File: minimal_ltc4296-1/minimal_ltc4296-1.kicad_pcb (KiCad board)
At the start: 4 copper layers, 71.1 x 53.3 mm, 44 parts, among them J1 TBP02R1-381-03BE, J2 TBP02R1-381-03BE, J3 TBP02R1-381-03BE, J4 TBP02R1-381-03BE, J5 TBP02R1-381-03BE, J6 TBP02R1-381-02BE, Q1 100.0 V, Q2 100.0 V, Q3 100.0 V, Q4 100.0 V, Q5 100.0 V, Q6 100.0 V, U1 LTC4296AUK-1-PBF

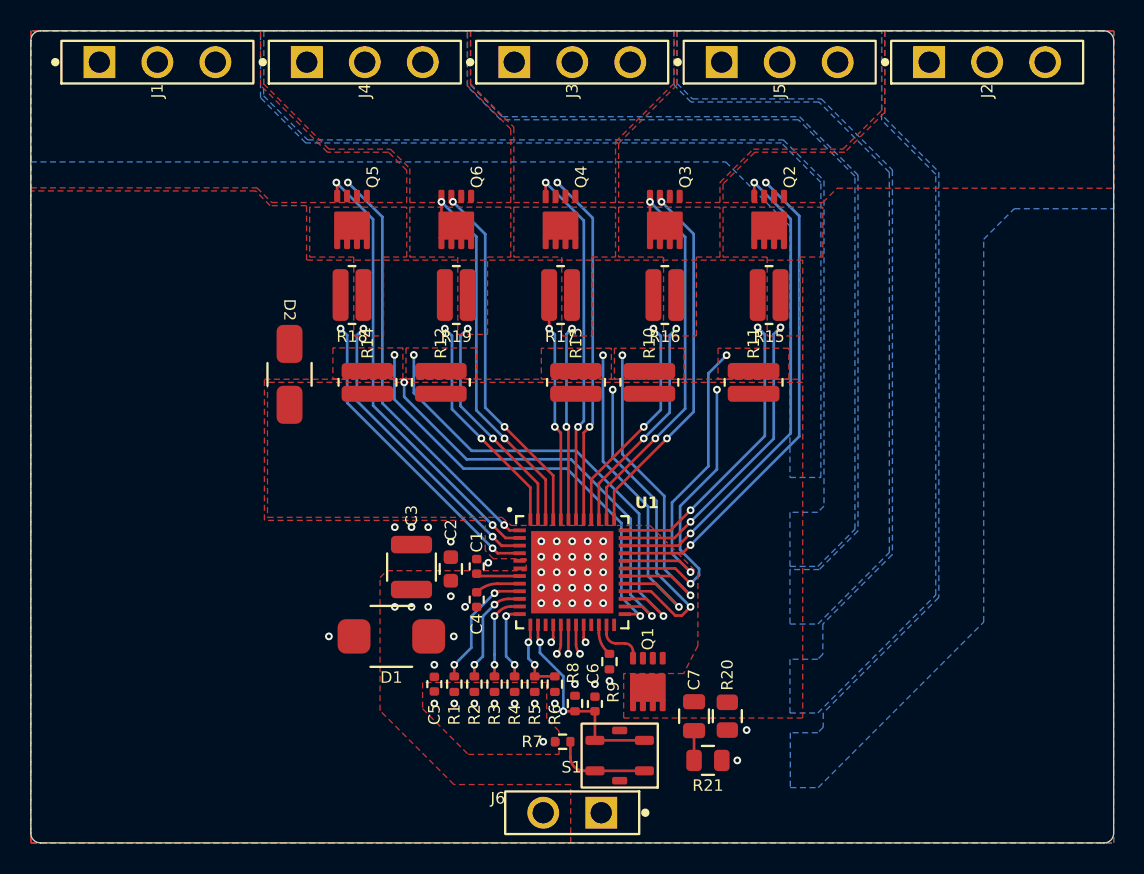
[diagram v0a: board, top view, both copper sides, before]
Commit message: Update KiCad PCB file
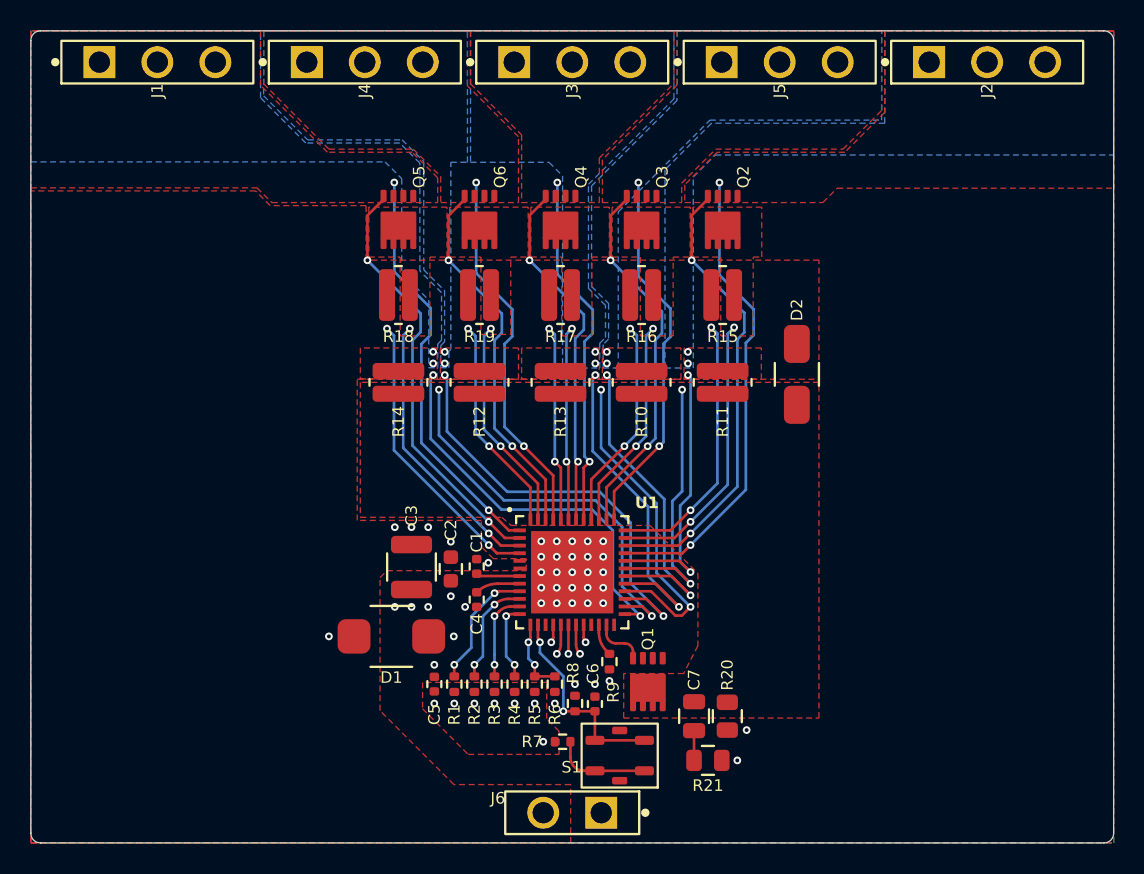
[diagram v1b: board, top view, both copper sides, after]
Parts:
- moved D2 33.3 mm to (164.5, 89.4)
- moved Q2 3.05 mm to (159.6, 79.2)
- moved Q5 3.05 mm to (138.3, 79.2)
- moved R15 3.05 mm to (159.6, 84.2)
- moved R18 3.05 mm to (138.3, 84.2)
- moved R12 2.54 mm to (143.6, 89.9)
- moved R11 2.03 mm to (159.6, 89.9)
- moved R14 2.03 mm to (138.3, 89.9)
- moved Q3 1.52 mm to (154.3, 79.2)
- moved Q6 1.52 mm to (143.6, 79.2)
- moved R16 1.52 mm to (154.3, 84.2)
- moved R19 1.52 mm to (143.6, 84.2)
- moved R13 1.02 mm to (148.9, 89.9)
- moved R10 0.51 mm to (154.3, 89.9)
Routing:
- net /PSE: track 84.1 -> 78.1 mm
- net /OUTM0: track 28.9 -> 26.1 mm, vias 2 -> 4
- net /OUTM4: track 20.9 -> 18.2 mm, vias 2 -> 4
- net /OUTM1: track 31.0 -> 28.3 mm, vias 2 -> 4
- net /LSNS: track 69.0 -> 66.4 mm
- net /HGATE4: track 32.3 -> 30.1 mm
- net /HGATE0: track 29.8 -> 28.1 mm
- net /HSNSM4: track 20.0 -> 18.7 mm
- net /HSNSM0: track 19.6 -> 18.3 mm
- net /OUTP4: track 32.2 -> 31.0 mm
- net /OUTP1: track 23.6 -> 24.7 mm
- net /OUTM2: track 22.8 -> 21.8 mm, vias 2 -> 4
- net /OUTM3: track 22.5 -> 21.6 mm, vias 2 -> 4
- net /HGATE2: track 24.3 -> 23.5 mm
- net /OUTP0: track 27.9 -> 27.2 mm
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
